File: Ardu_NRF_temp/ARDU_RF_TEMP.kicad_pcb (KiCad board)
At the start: 2 copper layers, 92 x 67 mm, 54 parts, among them J1 DE9_Pins, J2 Conn_01x04_Socket, J3 Conn_01x04_Socket, J4 Conn_01x04_Socket, SW2 SW_Push, SW3 SW_Push, U1 NRF24L01_Breakout, U2 DHT11, U3 ESP-WROOM-32D, U4 NRF24L01_Breakout

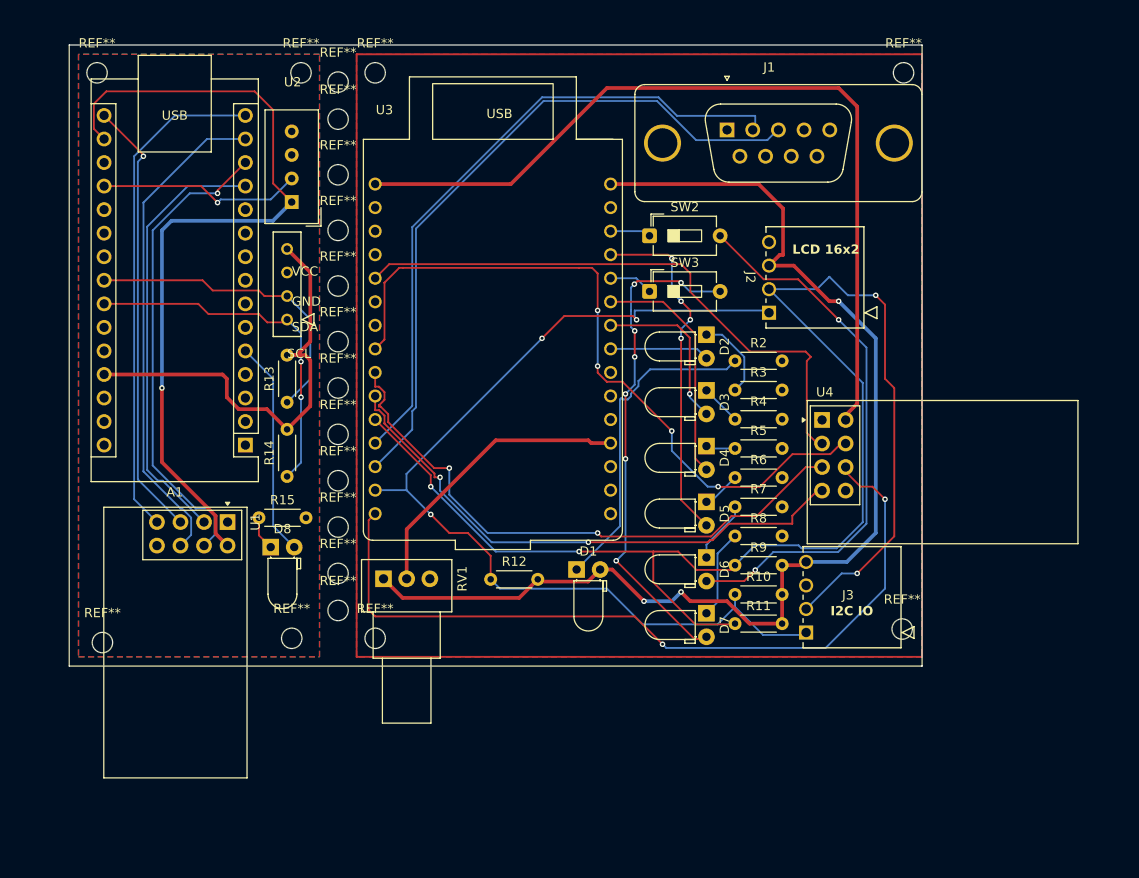
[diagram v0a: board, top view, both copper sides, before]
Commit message: 5/21/25-1
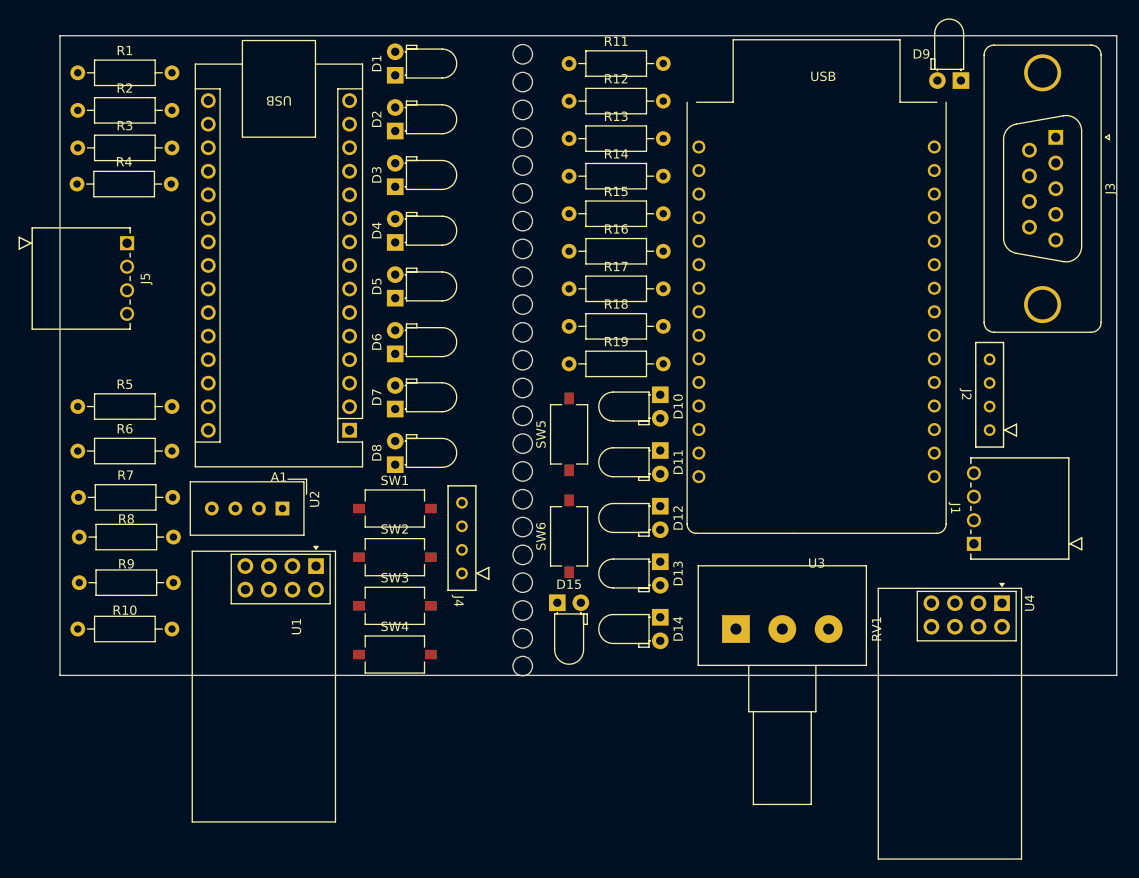
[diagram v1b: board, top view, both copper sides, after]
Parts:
- removed REF** (x20): MountingHole_2.2mm_M2, MountingHole:MountingHole_2.2mm_M2
- added ?: , , F.Cu at (61.9, 62.0)
- added ?: , , F.Cu at (61.9, 41.0)
- added ?: , , F.Cu at (61.9, 80.0)
- added ?: , , F.Cu at (61.9, 20.0)
- added ?: , , F.Cu at (61.9, 53.0)
- added ?: , , F.Cu at (61.9, 65.0)
- added ?: , , F.Cu at (61.9, 38.0)
- added ?: , , F.Cu at (61.9, 35.0)
- added ?: , , F.Cu at (61.9, 56.0)
- added ?: , , F.Cu at (61.9, 32.0)
- added ?: , , F.Cu at (61.9, 50.0)
- added ?: , , F.Cu at (61.9, 68.0)
- added ?: , , F.Cu at (61.9, 29.0)
- added ?: , , F.Cu at (61.9, 71.0)
- added ?: , , F.Cu at (61.9, 23.0)
- added ?: , , F.Cu at (61.9, 77.0)
- added ?: , , F.Cu at (61.9, 26.0)
- added ?: , , F.Cu at (61.9, 14.0)
- added ?: , , F.Cu at (61.9, 59.0)
- added ?: , , F.Cu at (61.9, 17.0)
- added ?: , , F.Cu at (61.9, 47.0)
- added ?: , , F.Cu at (61.9, 74.0)
- added ?: , , F.Cu at (61.9, 44.0)
- added D10: LED, LED_THT:LED_D3.0mm_Horizontal_O1.27mm_Z2.0mm, F.Cu at (76.8, 50.7)
- added D11: LED, LED_THT:LED_D3.0mm_Horizontal_O1.27mm_Z2.0mm, F.Cu at (76.8, 56.7)
- added D12: LED, LED_THT:LED_D3.0mm_Horizontal_O1.27mm_Z2.0mm, F.Cu at (76.8, 62.8)
- added D13: LED, LED_THT:LED_D3.0mm_Horizontal_O1.27mm_Z2.0mm, F.Cu at (76.8, 68.7)
- added D14: LED, LED_THT:LED_D3.0mm_Horizontal_O1.27mm_Z2.0mm, F.Cu at (76.8, 74.7)
- added D15: LED, LED_THT:LED_D3.0mm_Horizontal_O1.27mm_Z2.0mm, F.Cu at (65.7, 73.2)
- added D9: LED, LED_THT:LED_D3.0mm_Horizontal_O1.27mm_Z2.0mm, F.Cu at (109.2, 16.8)
- added J5: Conn_01x04_Socket, Add_New:CONN_PPPC041LGBN-RC_SUL, F.Cu at (19.2, 34.4)
- added R1: 3.3K, Resistor_THT:R_Axial_DIN0207_L6.3mm_D2.5mm_P10.16mm_Horizontal, F.Cu at (13.9, 16.0)
- added R16: 3.3K, Resistor_THT:R_Axial_DIN0207_L6.3mm_D2.5mm_P10.16mm_Horizontal, F.Cu at (66.9, 35.2)
- added R17: 3.3K, Resistor_THT:R_Axial_DIN0207_L6.3mm_D2.5mm_P10.16mm_Horizontal, F.Cu at (66.9, 39.3)
- added R18: 3.3K, Resistor_THT:R_Axial_DIN0207_L6.3mm_D2.5mm_P10.16mm_Horizontal, F.Cu at (66.9, 43.4)
- added R19: 3.3K, Resistor_THT:R_Axial_DIN0207_L6.3mm_D2.5mm_P10.16mm_Horizontal, F.Cu at (66.9, 47.4)
- added SW1: SW_Push, Button_Switch_SMD:SW_Tactile_SPST_NO_Straight_CK_PTS636Sx25SMTRLFS, F.Cu at (48.1, 63.0)
- added SW4: SW_Push, Button_Switch_SMD:SW_Tactile_SPST_NO_Straight_CK_PTS636Sx25SMTRLFS, F.Cu at (48.1, 78.8)
- added SW5: SW_Push, Button_Switch_SMD:SW_Tactile_SPST_NO_Straight_CK_PTS636Sx25SMTRLFS, F.Cu at (66.9, 55.0)
- added SW6: SW_Push, Button_Switch_SMD:SW_Tactile_SPST_NO_Straight_CK_PTS636Sx25SMTRLFS, F.Cu at (66.9, 66.0)
- J1: value DE9_Pins -> Conn_01x04_Socket; footprint Connector_Dsub:DSUB-9_Pins_Vertical_P2.77x2.84mm_MountingHoles -> Add_New:CONN_PPPC041LGBN-RC_SUL
- J2: footprint Add_New:CONN_PPPC041LGBN-RC_SUL -> Add_New:CONN_PPTC041LFBN-RC_SUL
- J3: value Conn_01x04_Socket -> DE9_Pins; footprint Add_New:CONN_PPPC041LGBN-RC_SUL -> Connector_Dsub:DSUB-9_Pins_Vertical_P2.77x2.84mm_MountingHoles
- R10, R12, R13, R15, R2, R3, R4, R5, R6, R7, R8, R9: footprint Resistor_THT:R_Axial_DIN0204_L3.6mm_D1.6mm_P5.08mm_Horizontal -> Resistor_THT:R_Axial_DIN0207_L6.3mm_D2.5mm_P10.16mm_Horizontal
- R11, R14: value 10K -> 3.3K; footprint Resistor_THT:R_Axial_DIN0204_L3.6mm_D1.6mm_P5.08mm_Horizontal -> Resistor_THT:R_Axial_DIN0207_L6.3mm_D2.5mm_P10.16mm_Horizontal
- RV1: footprint Potentiometer_THT:Potentiometer_Alps_RK09Y11_Single_Horizontal -> Potentiometer_THT:Potentiometer_Alps_RK163_Single_Horizontal
- SW2, SW3: footprint Button_Switch_THT:SW_DIP_SPSTx01_Slide_6.7x4.1mm_W7.62mm_P2.54mm_LowProfile -> Button_Switch_SMD:SW_Tactile_SPST_NO_Straight_CK_PTS636Sx25SMTRLFS
- moved R2 75.9 mm to (13.9, 20.1)
- moved R3 75.6 mm to (13.9, 24.1)
- moved R4 75.4 mm to (13.8, 28.0)
- moved R5 71.0 mm to (13.9, 52.0)
- moved R10 71.0 mm to (13.9, 76.0)
- moved R6 71.0 mm to (13.9, 56.8)
- moved R7 70.8 mm to (14.0, 61.8)
- moved R9 70.8 mm to (14.1, 71.0)
- moved R8 70.7 mm to (14.1, 66.1)
- moved R11 63.0 mm to (66.9, 15.0)
- moved J3 59.8 mm to (119.4, 23.0)
- moved D1 56.8 mm to (48.2, 16.3), turned to 90 degrees
- moved R12 52.3 mm to (66.9, 19.1)
- moved J1 52.0 mm to (110.6, 66.8), turned to -90 degrees
- moved R15 46.9 mm to (66.9, 31.2)
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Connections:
- A1 pad 1: unconnected-(A1-D1/TX-Pad1) -> Net-(A1-D1/TX)
- A1 pad 10: unconnected-(A1-D7-Pad10) -> Net-(A1-D7)
- A1 pad 11: unconnected-(A1-D8-Pad11) -> Net-(A1-D8)
- A1 pad 17: 3V3 -> 3V31
- A1 pad 2: unconnected-(A1-D0/RX-Pad2) -> Net-(A1-D0/RX)
- A1 pad 6: unconnected-(A1-D3-Pad6) -> Net-(A1-D3)
- A1 pad 8: unconnected-(A1-D5-Pad8) -> Net-(A1-D5)
- A1 pad 9: unconnected-(A1-D6-Pad9) -> Net-(A1-D6)
- D1 pad 1: Net-(D1-K) -> GND1
- D1 pad 2: VCC -> Net-(D1-A)
- D2 pad 1: Net-(D2-K) -> GND1
- D2 pad 2: GPIO25 -> Net-(D2-A)
- D3 pad 1: Net-(D3-K) -> GND1
- D3 pad 2: GPIO26 -> Net-(D3-A)
- D4 pad 1: Net-(D4-K) -> GND1
- D4 pad 2: GPIO27 -> Net-(D4-A)
- D5 pad 2: GPIO12 -> Net-(A1-D5)
- D6 pad 2: Net-(D6-A) -> Net-(A1-D6)
- D7 pad 2: Net-(D7-A) -> Net-(A1-D7)
- D8 pad 2: Net-(A1-D2) -> Net-(A1-D8)
- J1 pad 1: unconnected-(J1-Pad1) -> SCL
- J1 pad 2: Net-(U3-RXD0/IO3) -> SDA
- J1 pad 3: Net-(U3-TXD0/IO1) -> VCC
- J1 pad 4: unconnected-(J1-Pad4) -> GND
- J2 pad 3: VCC -> GND
- J2 pad 4: GND -> VCC
- J3 pad 1: SCL -> unconnected-(J3-Pad1)
- J3 pad 2: SDA -> Net-(U3-RXD0/IO3)
- J3 pad 3: GND -> Net-(U3-TXD0/IO1)
- J3 pad 4: VCC -> unconnected-(J3-Pad4)
- R10 pad 1: SCL -> SDA1
- R10 pad 2: VCC -> GND1
- R11 pad 1: SDA -> Net-(D9-K)
- R11 pad 2: VCC -> GND
- R12 pad 1: SCL -> GND
- R12 pad 2: VCC -> SCL
- R13 pad 1: SDA1 -> GND
- R13 pad 2: VCC1 -> SDA
- R14 pad 1: SCL1 -> 3V3
- R14 pad 2: VCC1 -> GPIO13
- R15 pad 1: Net-(D8-K) -> 3V3
- R15 pad 2: GND1 -> GPIO14
- R2 pad 1: Net-(D1-K) -> Net-(D6-K)
- R2 pad 2: GND -> GND1
- R3 pad 1: Net-(D2-K) -> Net-(D7-K)
- R3 pad 2: GND -> GND1
- R4 pad 1: Net-(D3-K) -> Net-(D8-K)
- R4 pad 2: GND -> GND1
- R5 pad 1: Net-(D4-K) -> VCC1
- R5 pad 2: GND -> Net-(A1-D3)
- R6 pad 1: Net-(D5-K) -> VCC1
- R6 pad 2: GND -> Net-(A1-D2)
- R7 pad 1: Net-(D6-K) -> VCC1
- R7 pad 2: GND -> Net-(A1-D1/TX)
- R8 pad 1: Net-(D7-K) -> VCC1
- R8 pad 2: GND -> Net-(A1-D0/RX)
- R9 pad 1: SDA -> SCL1
- R9 pad 2: VCC -> GND1
- SW2 pad 1: GPIO13 -> Net-(D2-A)
- SW2 pad 2: Net-(D6-A) -> Net-(A1-D1/TX)
- SW3 pad 1: GPIO14 -> Net-(D3-A)
- SW3 pad 2: Net-(D7-A) -> Net-(A1-D2)
- U1 pad 2: 3V3 -> 3V31
- U2 pad 1: 3V3 -> 3V31
- U3 pad 16: Net-(U3-3V3) -> unconnected-(U3-3V3-Pad16)
- U4 pad 2: Net-(U3-3V3) -> 3V3
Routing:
- net SDA: track 158.3 -> 0.00 mm, vias 4 -> 0
- net VCC: track 128.8 -> 0.00 mm, vias 3 -> 0
- net SCL: track 106.9 -> 0.00 mm, vias 3 -> 0
- net Net-(U3-3V3): track 91.7 -> 0.00 mm
- net 3V3: track 87.9 -> 0.00 mm, vias 1 -> 0
- net MOSI1: track 86.5 -> 0.00 mm, vias 2 -> 0
- net CSN1: track 76.7 -> 0.00 mm, vias 4 -> 0
- net Net-(U3-TXD0/IO1): track 74.4 -> 0.00 mm
- net Net-(U3-RXD0/IO3): track 70.3 -> 0.00 mm
- net SCK1: track 63.0 -> 0.00 mm, vias 2 -> 0
- net CE1: track 63.0 -> 0.00 mm
- net Net-(D6-A): track 59.6 -> 0.00 mm, vias 2 -> 0
- net MISO1: track 59.5 -> 0.00 mm, vias 2 -> 0
- net MISO: track 54.3 -> 0.00 mm
- net Net-(D7-A): track 54.2 -> 0.00 mm, vias 7 -> 0
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- removed copper zone on B.Cu, net GND
- removed copper zone on F.Cu, net GND
- removed copper zone on B.Cu, net GND1
- removed copper zone on F.Cu, net GND1
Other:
- board size 92 x 67 mm -> 114 x 69 mm
- board text added: "Ohguk Kwon"
- board text removed: "GND"
- board text removed: "I2C IO"
- board text removed: "LCD 16x2"
- board text removed: "SCL"
- board text removed: "SDA"
- board text removed: "VCC"
